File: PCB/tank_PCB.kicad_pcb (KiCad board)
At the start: 2 copper layers, 49 x 91 mm, 64 parts, among them J1 TFT, J2 PTSA 1,5/ 2-3,5-Z, J3 PTSA 1,5/ 8-3,5-Z, J5 USB4110GFA, U1 ADS1115IDGS, U3 LM2735X (1.6MHz), U4 ESP32-C6-WROOM-1, U5 MCP1826S-3302E/DB

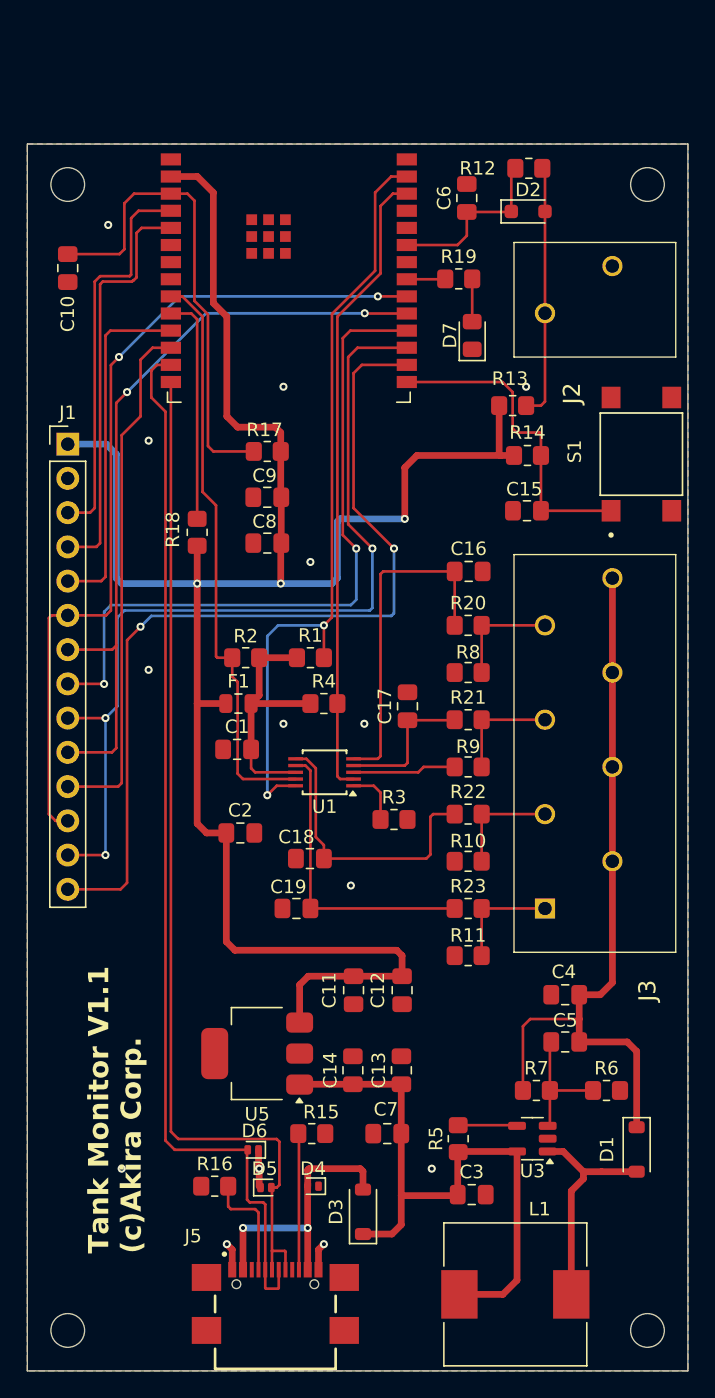
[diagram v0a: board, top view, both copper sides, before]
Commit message: Clearing Kicad Warnings
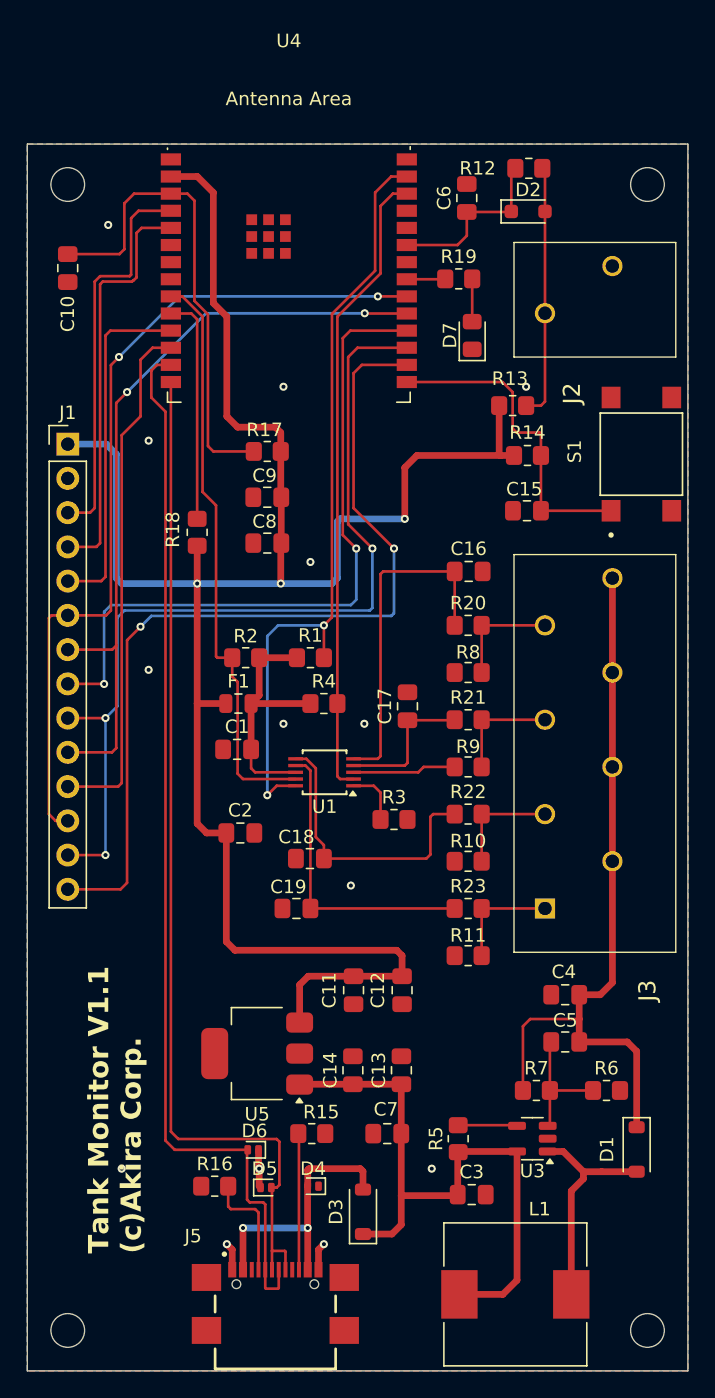
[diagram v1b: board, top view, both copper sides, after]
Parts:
- U4: footprint PCM_Espressif:ESP32-C6-WROOM-1 -> zTankFootprints:ESP32-C6-WROOM-1
